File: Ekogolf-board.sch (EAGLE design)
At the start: 10 parts

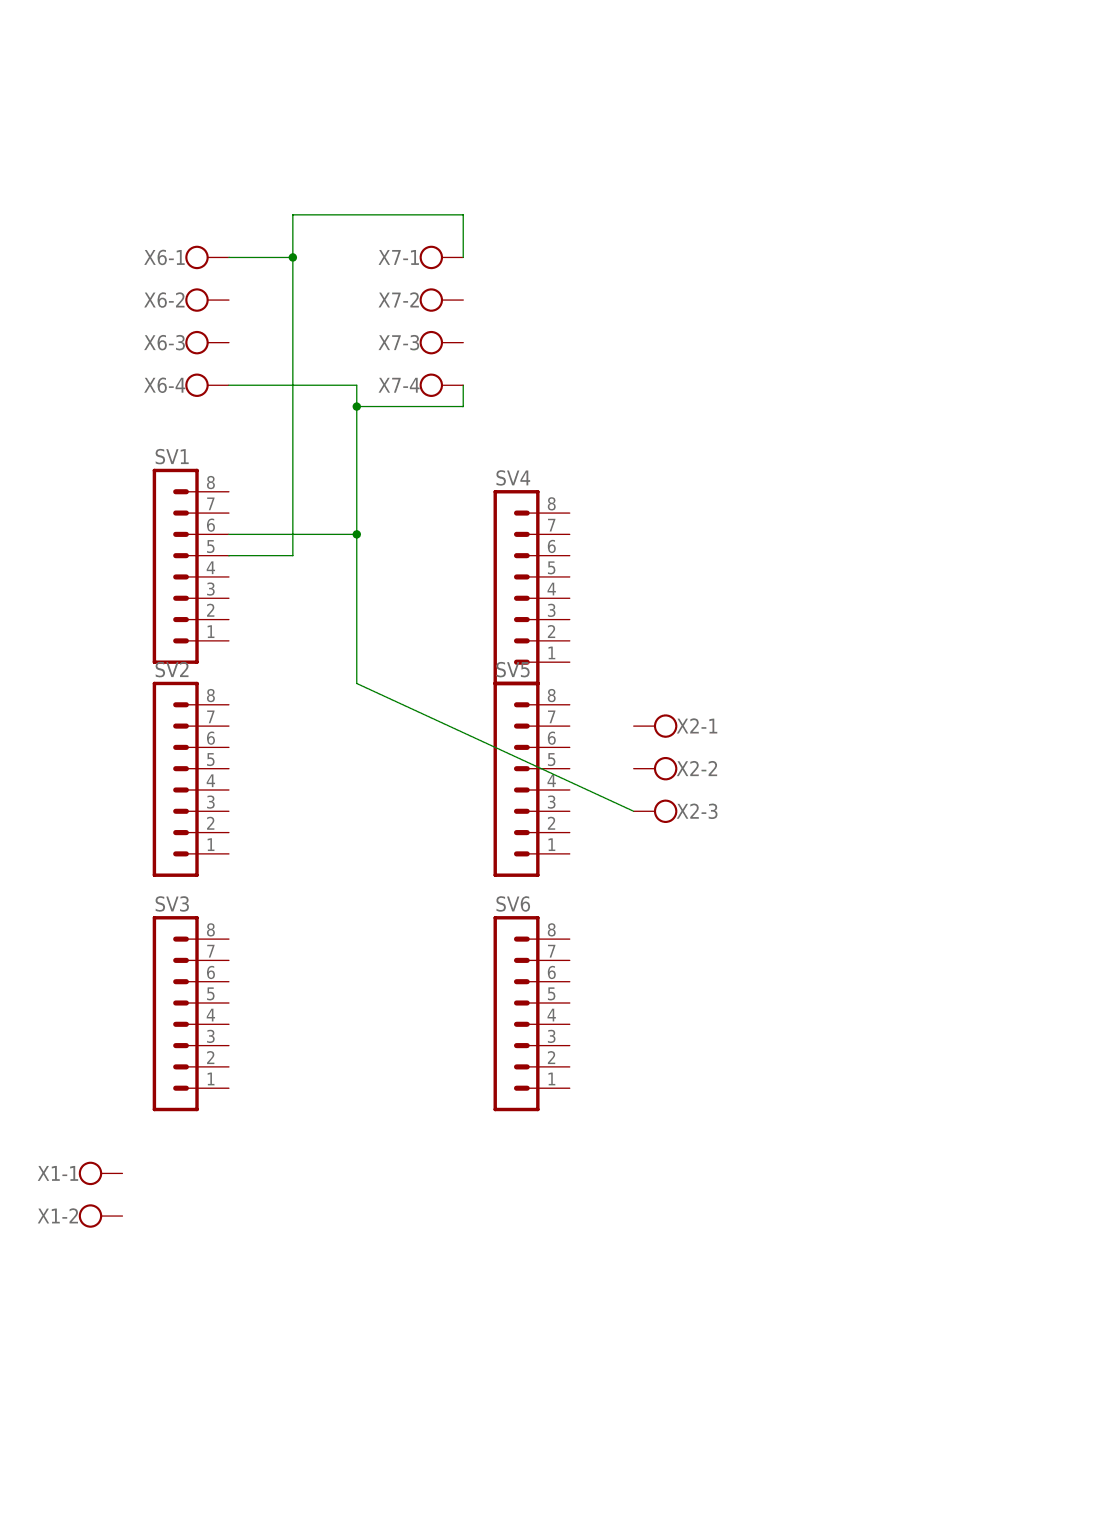
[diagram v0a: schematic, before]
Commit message: Poligono de Masa a GND
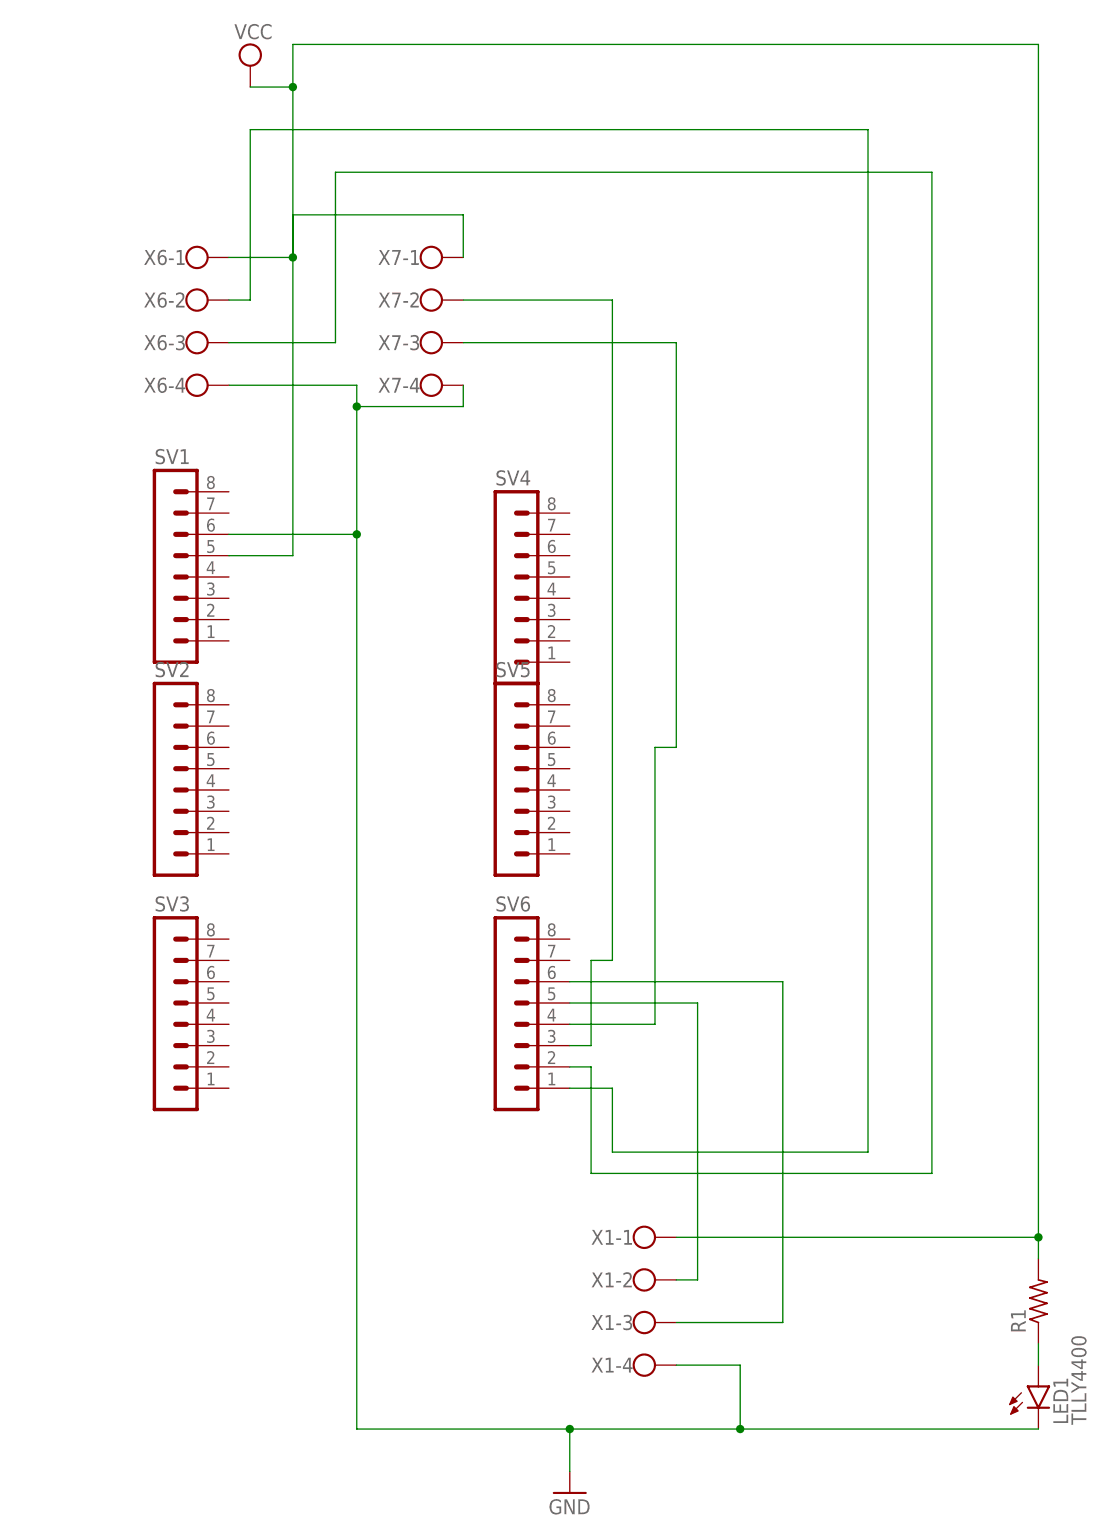
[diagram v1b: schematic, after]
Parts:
- removed X2: (no value), con-wago-500:W237-103
- added LED1: TLLY4400, led:TLLY4400
- added R1: (no value), rcl:R-US_0204/5
- X1: device con-wago-500:W237-102 -> con-wago-500:W237-4
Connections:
- removed net N$3: SV1.6, X2-3.KL, X6-4.KL, X7-4.KL
- new net GND: LED1.C, SV1.6, X1-4.KL, X6-4.KL, X7-4.KL
- new net N$10: SV6.5, X1-2.KL
- new net N$5: SV6.4, X7-3.KL
- new net N$6: SV6.3, X7-2.KL
- new net N$7: SV6.2, X6-3.KL
- new net N$9: SV6.6, X1-3.KL
- new net TX3: SV6.1, X6-2.KL
- new net VCC: R1.2, SV1.5, X1-1.KL, X6-1.KL, X7-1.KL
- net N$1: now also LED1.A, R1.1; no longer SV1.5, X6-1.KL, X7-1.KL
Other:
- moved on the sheet: X1-1, X1-2
